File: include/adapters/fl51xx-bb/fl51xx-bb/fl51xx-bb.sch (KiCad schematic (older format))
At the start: 3 parts, among them J1 Conn_01x05, J2 Conn_01x05, U1 FL51xxMX

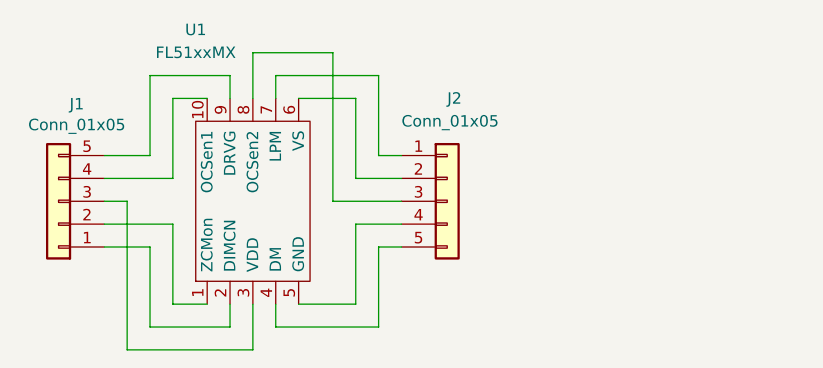
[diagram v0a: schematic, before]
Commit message: first order
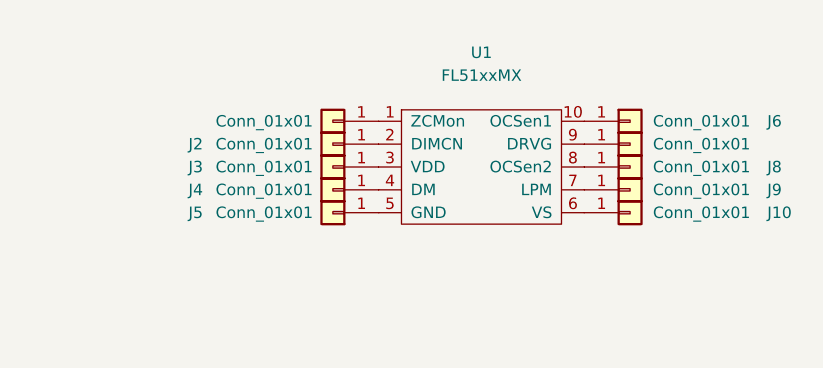
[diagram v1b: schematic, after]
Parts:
- removed J1, J2: Conn_01x05, Connector_PinHeader_2.54mm:PinHeader_1x05_P2.54mm_Vertical, symbol Connector_Generic:Conn_01x05
- added J1, J10, J2, J3, J4, J5, J6, J7, J8, J9: Conn_01x01, Connector_PinHeader_2.54mm:PinHeader_1x01_P2.54mm_Vertical, symbol Connector_Generic:Conn_01x01
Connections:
- net at U1.1 (ZCMon): now also J1.1 (Pin_1)
- net at U1.10 (OCSen1): now also J6.1 (Pin_1)
- net at U1.2 (DIMCN): now also J2.1 (Pin_1)
- net at U1.3 (VDD): now also J3.1 (Pin_1)
- net at U1.4 (DM): now also J4.1 (Pin_1)
- net at U1.5 (GND): now also J5.1 (Pin_1)
- net at U1.6 (VS): now also J10.1 (Pin_1)
- net at U1.7 (LPM): now also J9.1 (Pin_1)
- net at U1.8 (OCSen2): now also J8.1 (Pin_1)
- net at U1.9 (DRVG): now also J7.1 (Pin_1)
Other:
- moved on the sheet: U1
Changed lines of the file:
@@
 EESchema Schematic File Version 4
+LIBS:fl51xx-bb-cache
 EELAYER 26 0
 EELAYER END
-$Descr A4 11693 8268
+$Descr User 5197 4000
 encoding utf-8
 Sheet 1 1
-Title ""
-Date ""
-Rev ""
-Comp ""
+Title "FL51xx BREADBOARD ADAPTER"
+Date "2019-10-07"
+Rev "v1.0.0"
+Comp "slimc"
 Comment1 ""
 Comment2 ""
@@
 L AC_Drivers:FL51xxMX U1
 U 1 1 5DAD29E3
-P 1550 1400
-F 0 "U1" V 2300 1650 50  0000 C CNN
-F 1 "FL51xxMX" V 2200 1650 50  0000 C CNN
-F 2 "AC_Drivers:FL51xxMX" H 1200 1800 50  0001 C CNN
-F 3 "" H 1200 1800 50  0001 C CNN
-	1    1550 1400
-	0    -1   -1   0
-$EndComp
-$Comp
-L Connector_Generic:Conn_01x05 J2
-U 1 1 5DAD3048
-P 2400 1400
-F 0 "J2" H 2400 1850 50  0000 L CNN
-F 1 "Conn_01x05" H 2200 1750 50  0000 L CNN
-F 2 "Connector_PinHeader_2.54mm:PinHeader_1x05_P2.54mm_Vertical" H 2400 1400 50  0001 C CNN
-F 3 "~" H 2400 1400 50  0001 C CNN
-	1    2400 1400
+P 2550 1250
+F 0 "U1" H 2550 1750 50  0000 C CNN
+F 1 "FL51xxMX" H 2550 1650 50  0000 C CNN
+F 2 "AC_Drivers:FL51xxMX" H 2200 1650 50  0001 C CNN
+F 3 "" H 2200 1650 50  0001 C CNN
+	1    2550 1250
 	1    0    0    -1
 $EndComp
 $Comp
-L Connector_Generic:Conn_01x05 J1
-U 1 1 5DAD3118
-P 700 1400
-F 0 "J1" H 620 975 50  0000 C CNN
-F 1 "Conn_01x05" H 620 1066 50  0000 C CNN
-F 2 "Connector_PinHeader_2.54mm:PinHeader_1x05_P2.54mm_Vertical" H 700 1400 50  0001 C CNN
-F 3 "~" H 700 1400 50  0001 C CNN
-	1    700  1400
+L Connector_Generic:Conn_01x01 J6
+U 1 1 5D9B2700
+P 3200 1050
+F 0 "J6" H 3800 1050 50  0000 L CNN
+F 1 "Conn_01x01" H 3300 1050 50  0000 L CNN
+F 2 "Connector_PinHeader_2.54mm:PinHeader_1x01_P2.54mm_Vertical" H 3200 1050 50  0001 C CNN
+F 3 "~" H 3200 1050 50  0001 C CNN
+	1    3200 1050
+	1    0    0    -1
+$EndComp
+$Comp
+L Connector_Generic:Conn_01x01 J1
+U 1 1 5D9B2AB1
+P 1900 1050
+F 0 "J1" H 2500 1050 50  0001 C CNN
+F 1 "Conn_01x01" H 2200 1050 50  0000 C CNN
+F 2 "Connector_PinHeader_2.54mm:PinHeader_1x01_P2.54mm_Vertical" H 1900 1050 50  0001 C CNN
+F 3 "~" H 1900 1050 50  0001 C CNN
+	1    1900 1050
 	-1   0    0    1
 $EndComp
-Wire Wire Line
-	1350 1850 1200 1850
-Wire Wire Line
-	1200 1850 1200 1500
-Wire Wire Line
-	1200 1500 900  1500
-Wire Wire Line
-	1450 1850 1450 1950
-Wire Wire Line
-	1450 1950 1100 1950
-Wire Wire Line
-	1100 1950 1100 1600
-Wire Wire Line
-	1100 1600 900  1600
-Wire Wire Line
-	1550 1850 1550 2050
-Wire Wire Line
-	1550 2050 1000 2050
-Wire Wire Line
-	1000 2050 1000 1400
-Wire Wire Line
-	1000 1400 900  1400
-Wire Wire Line
-	1350 950  1200 950
-Wire Wire Line
-	1200 950  1200 1300
-Wire Wire Line
-	1200 1300 900  1300
-Wire Wire Line
-	1450 950  1450 850
-Wire Wire Line
-	1450 850  1100 850
-Wire Wire Line
-	1100 850  1100 1200
-Wire Wire Line
-	1100 1200 900  1200
-Wire Wire Line
-	1750 1850 2000 1850
-Wire Wire Line
-	2000 1850 2000 1500
-Wire Wire Line
-	2000 1500 2200 1500
-Wire Wire Line
-	1650 1850 1650 1950
-Wire Wire Line
-	1650 1950 2100 1950
-Wire Wire Line
-	2100 1950 2100 1600
-Wire Wire Line
-	2100 1600 2200 1600
-Wire Wire Line
-	1750 950  2000 950
-Wire Wire Line
-	2000 950  2000 1300
-Wire Wire Line
-	2000 1300 2200 1300
-Wire Wire Line
-	1650 950  1650 850
-Wire Wire Line
-	1650 850  2100 850
-Wire Wire Line
-	2100 850  2100 1200
-Wire Wire Line
-	2100 1200 2200 1200
-Wire Wire Line
-	1550 950  1550 750
-Wire Wire Line
-	1550 750  1900 750
-Wire Wire Line
-	1900 750  1900 1400
-Wire Wire Line
-	1900 1400 2200 1400
+$Comp
+L Connector_Generic:Conn_01x01 J2
+U 1 1 5D9B2B7D
+P 1900 1150
+F 0 "J2" H 2500 1150 50  0000 C CNN
+F 1 "Conn_01x01" H 2200 1150 50  0000 C CNN
+F 2 "Connector_PinHeader_2.54mm:PinHeader_1x01_P2.54mm_Vertical" H 1900 1150 50  0001 C CNN
+F 3 "~" H 1900 1150 50  0001 C CNN
+	1    1900 1150
+	-1   0    0    1
+$EndComp
+$Comp
+L Connector_Generic:Conn_01x01 J3
+U 1 1 5D9B2BA9
+P 1900 1250
+F 0 "J3" H 2500 1250 50  0000 C CNN
+F 1 "Conn_01x01" H 2200 1250 50  0000 C CNN
+F 2 "Connector_PinHeader_2.54mm:PinHeader_1x01_P2.54mm_Vertical" H 1900 1250 50  0001 C CNN
+F 3 "~" H 1900 1250 50  0001 C CNN
+	1    1900 1250
+	-1   0    0    1
+$EndComp
+$Comp
+L Connector_Generic:Conn_01x01 J4
+U 1 1 5D9B2BCF
+P 1900 1350
+F 0 "J4" H 2500 1350 50  0000 C CNN
+F 1 "Conn_01x01" H 2200 1350 50  0000 C CNN
+F 2 "Connector_PinHeader_2.54mm:PinHeader_1x01_P2.54mm_Vertical" H 1900 1350 50  0001 C CNN
+F 3 "~" H 1900 1350 50  0001 C CNN
+	1    1900 1350
+	-1   0    0    1
+$EndComp
+$Comp
+L Connector_Generic:Conn_01x01 J5
+U 1 1 5D9B2BF7
+P 1900 1450
+F 0 "J5" H 2500 1450 50  0000 C CNN
+F 1 "Conn_01x01" H 2200 1450 50  0000 C CNN
+F 2 "Connector_PinHeader_2.54mm:PinHeader_1x01_P2.54mm_Vertical" H 1900 1450 50  0001 C CNN
+F 3 "~" H 1900 1450 50  0001 C CNN
+	1    1900 1450
+	-1   0    0    1
+$EndComp
+$Comp
+L Connector_Generic:Conn_01x01 J7
+U 1 1 5D9B3066
+P 3200 1150
+F 0 "J7" H 3800 1150 50  0001 L CNN
+F 1 "Conn_01x01" H 3300 1150 50  0000 L CNN
+F 2 "Connector_PinHeader_2.54mm:PinHeader_1x01_P2.54mm_Vertical" H 3200 1150 50  0001 C CNN
+F 3 "~" H 3200 1150 50  0001 C CNN
+	1    3200 1150
+	1    0    0    -1
+$EndComp
+$Comp
+L Connector_Generic:Conn_01x01 J8
+U 1 1 5D9B3086
+P 3200 1250
+F 0 "J8" H 3800 1250 50  0000 L CNN
+F 1 "Conn_01x01" H 3300 1250 50  0000 L CNN
+F 2 "Connector_PinHeader_2.54mm:PinHeader_1x01_P2.54mm_Vertical" H 3200 1250 50  0001 C CNN
+F 3 "~" H 3200 1250 50  0001 C CNN
+	1    3200 1250
+	1    0    0    -1
+$EndComp
+$Comp
+L Connector_Generic:Conn_01x01 J9
+U 1 1 5D9B30A8
+P 3200 1350
+F 0 "J9" H 3800 1350 50  0000 L CNN
+F 1 "Conn_01x01" H 3300 1350 50  0000 L CNN
+F 2 "Connector_PinHeader_2.54mm:PinHeader_1x01_P2.54mm_Vertical" H 3200 1350 50  0001 C CNN
+F 3 "~" H 3200 1350 50  0001 C CNN
+	1    3200 1350
+	1    0    0    -1
+$EndComp
+$Comp
+L Connector_Generic:Conn_01x01 J10
+U 1 1 5D9B30D0
+P 3200 1450
+F 0 "J10" H 3800 1450 50  0000 L CNN
+F 1 "Conn_01x01" H 3300 1450 50  0000 L CNN
+F 2 "Connector_PinHeader_2.54mm:PinHeader_1x01_P2.54mm_Vertical" H 3200 1450 50  0001 C CNN
+F 3 "~" H 3200 1450 50  0001 C CNN
+	1    3200 1450
+	1    0    0    -1
+$EndComp
 $EndSCHEMATC
